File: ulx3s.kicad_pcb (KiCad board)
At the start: 4 copper layers, 94 x 50.8 mm, 222 parts, among them J1 CONN_02X20, J2 CONN_02X20, J3 WIFI_OFF, J4 CONN_02X03, J5 VJ1, Q1 BC857, Q2 2N7002, SW1 SW_DIP_x04, U1 LFE5U-85F-6BG381C, U10 IS25LP128F-JBLE, U11 PCA9306D, U2 MT48LC16M16A2TG, U3 TLV62569DBV, U4 TLV62569DBV, U5 TLV62569DBV, U6 FT231XS, U7 MCP7940NT, U8 MAX11125, U9 ESP32, Y1 FNETHE025, Y2 32768Hz

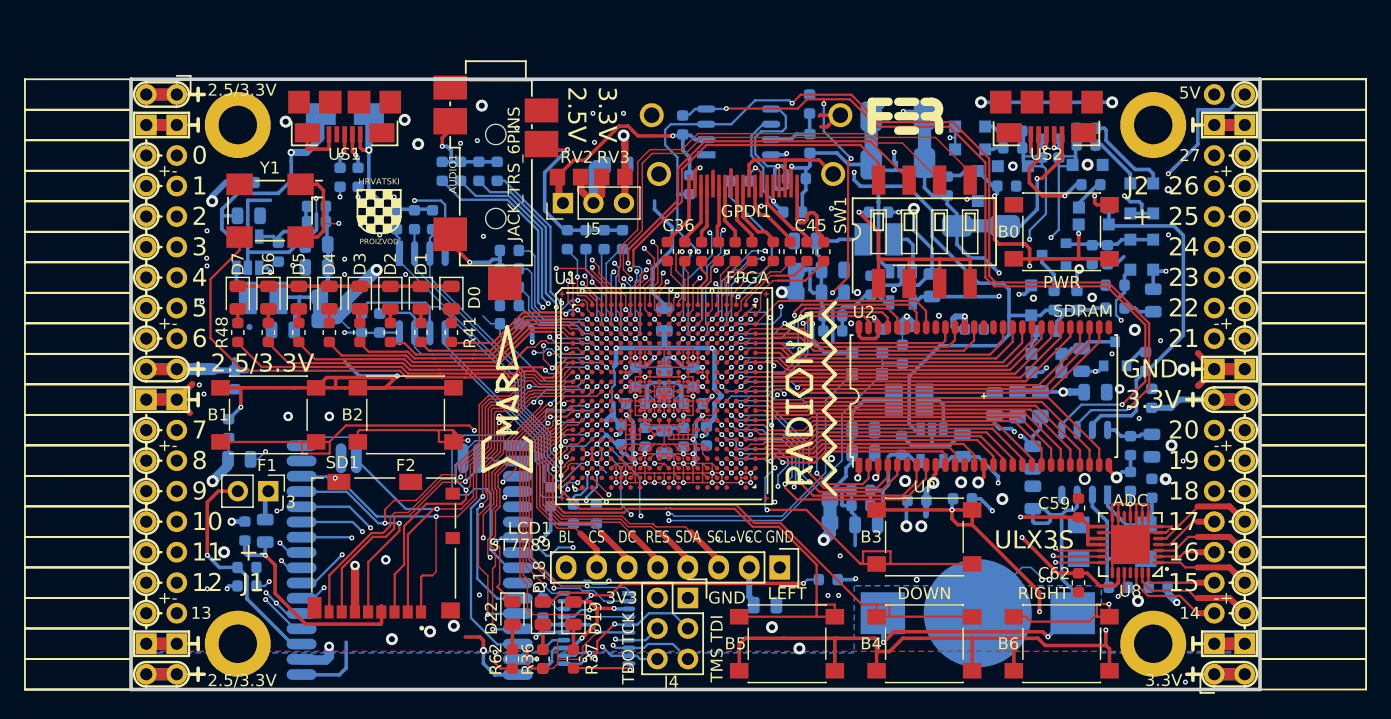
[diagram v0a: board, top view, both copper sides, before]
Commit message: First pass cleanup
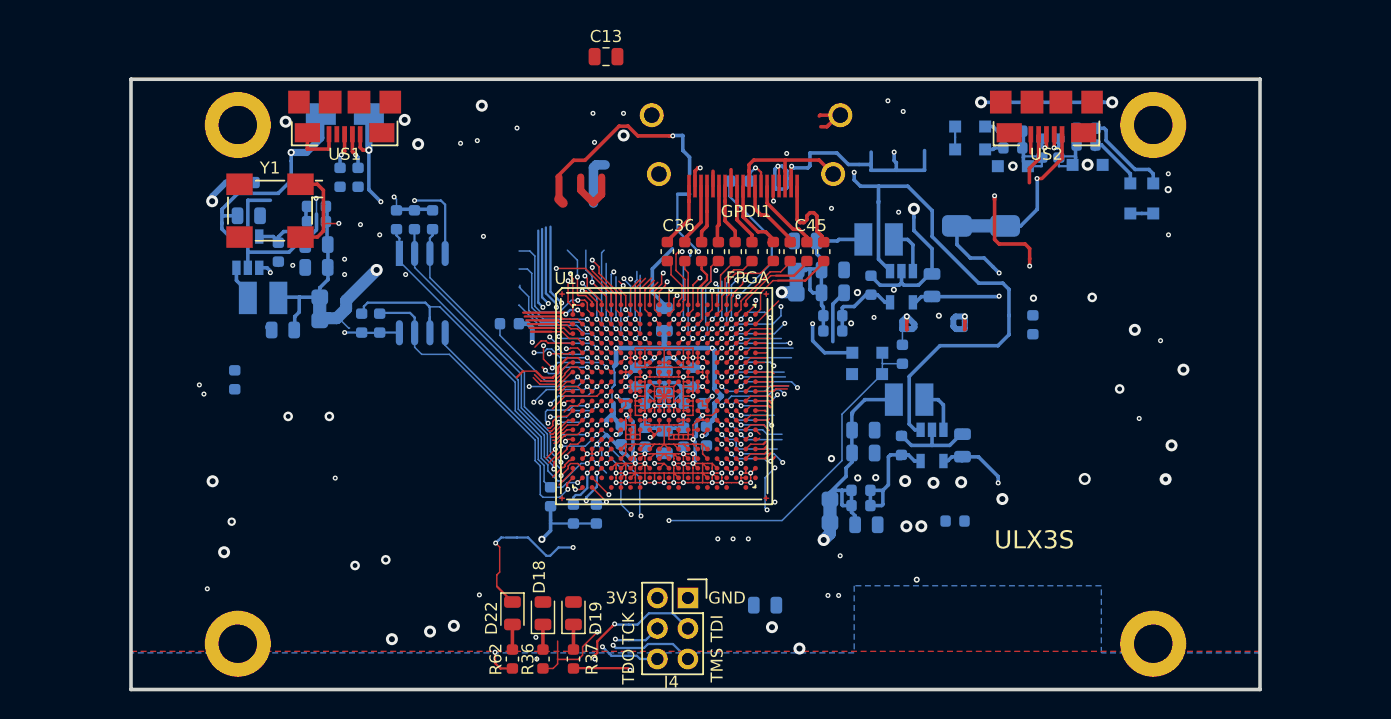
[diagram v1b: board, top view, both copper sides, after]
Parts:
- removed AE1: 433MHz, TestPoint:TestPoint_Pad_D1.0mm
- removed AUDIO1: JACK_TRS_6PINS, audio-jack:CUI_SJ-43516-SMT
- removed B0, B1, B2, B3, B4, B5, B6: PTS645, Button_Switch_SMD:SW_SPST_PTS645
- removed BAT1: CR1225, Keystone_3000_1x12mm-CoinCell:Keystone_3000_1x12mm-CoinCell
- removed C14, C59, C60, C62: 220nF, Capacitor_SMD:C_0603_1608Metric
- removed C15, C21, C54, C55, C58, C61: 22uF, Capacitor_SMD:C_0805_2012Metric
- removed C16, C47: 2.2uF, Capacitor_SMD:C_0805_2012Metric
- removed C18: 470pF, Capacitor_SMD:C_0603_1608Metric
- removed C33, C34, C35, C52: 22nF, Capacitor_SMD:C_0603_1608Metric
- removed C56, C57: 4.7pF, Capacitor_SMD:C_0603_1608Metric
- removed D0, D11, D4: RED, LED_SMD:LED_0805_2012Metric
- removed D1, D5: ORANGE, LED_SMD:LED_0805_2012Metric
- removed D10, D13, D14, D16, D17, D27: 1N914, Diode_SMD:D_SOD-323_HandSoldering
- removed D12, D15: BAT54W, Diode_SMD:D_SOD-323_HandSoldering
- removed D2, D6: GREEN, LED_SMD:LED_0805_2012Metric
- removed D3, D7: BLUE, LED_SMD:LED_0805_2012Metric
- removed D51, D52: 0, jumper:D_SMA_Jumper_NC
- removed HR: HR, hrvatski_proizvod_veci:hrvatski
- removed J1, J2: CONN_02X20, Socket_Strips:Socket_Strip_Angled_2x20
- removed J3: WIFI_OFF, Connector_PinHeader_2.54mm:PinHeader_1x02_P2.54mm_Vertical
- removed J5: VJ1, Connector_PinHeader_2.54mm:PinHeader_1x03_P2.54mm_Vertical
- removed L4, L5: 33uH, Inductor_SMD:L_0805_2012Metric_Pad1.15x1.40mm_HandSolder
- removed LCD1: ST7789, st7789:st7789
- removed Q1: BC857, Package_TO_SOT_SMD:SOT-23
- removed Q2: 2N7002, Package_TO_SOT_SMD:SOT-23
- removed R1, R25, R26, R3, R4: 4.7k, Resistor_SMD:R_0603_1608Metric
- removed R10, R17, R21, R39, R51, R60, R7: 130, Resistor_SMD:R_0603_1608Metric
- removed R13, R34, R9: 15k, Resistor_SMD:R_0603_1608Metric
- removed R14, R18, R57, R6, R66, R8: 1.1k, Resistor_SMD:R_0603_1608Metric
- removed R15, R19, R35, R41, R42, R43, R44, R45, R46, R47, R48, R58, R65: 549, Resistor_SMD:R_0603_1608Metric
- removed R16, R20, R59: 270, Resistor_SMD:R_0603_1608Metric
- removed R2: 18k, Resistor_SMD:R_0603_1608Metric
- removed R22, R23: 3.3k, Resistor_SMD:R_0603_1608Metric
- removed R24: 100k, Resistor_SMD:R_0603_1608Metric
- removed R38: 0.47, Resistor_SMD:R_0603_1608Metric
- removed R5: 2.2M, Resistor_SMD:R_0603_1608Metric
- removed R56: 0, Resistor_SMD:R_0603_1608Metric
- removed REF** (x2): emard12mm, emard:emard12mm
- removed REF**: inem, inem:inem
- removed RV2, RV3: 0, Resistor_SMD:R_0805_2012Metric_Pad1.29x1.40mm_HandSolder
- removed SD1: 104031-0811, micro-sd-104031-811:MOLEX_104031-0811
- removed SW1: SW_DIP_x04, dipswitch:SW_DIP_x4_W8.61mm_Slide_LowProfile
- removed U11: PCA9306D, SM8:SM8
- removed U2: MT48LC16M16A2TG, TSOP54:TSOP54
- removed U6: FT231XS, ft231x:FT231X-SSOP-20_4.4x6.5mm_Pitch0.65mm
- removed U7: MCP7940NT, SOT96-1:SOT96-1
- removed U8: MAX11125, max1112x-tqfn28:MAX1112x-TQFN-28-1EP_5x5mm_Pitch0.5mm
- removed U9: ESP32, ESP32:ESP32
- removed Y2: 32768Hz, abs25:Crystal_SMD_ABS25
- removed fer: fer, fer:fer
- removed koncar: koncar, koncar:koncar
- removed radiona: radiona, radiona:radiona
- C13: moved to F.Cu
- moved C13 46.9 mm to (133.6, 59.5), turned to 0 degrees
- moved C51 17.8 mm to (162.7, 98.2)
- moved C50 11.6 mm to (169.2, 81.9)
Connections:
- C13 pad 1: +5V -> GND
- C13 pad 2: /power/WKUP -> 2V5_3V3
- C20 pad 1: +3V3 -> 2V5_3V3
- C25 pad 1: +3V3 -> 2V5_3V3
- C31 pad 1: +3V3 -> 2V5_3V3
- C32 pad 1: +3V3 -> 2V5_3V3
- C46 pad 1: +3V3 -> 2V5_3V3
- C50 pad 1: +3V3 -> 2V5_3V3
- C51 pad 1: +3V3 -> 2V5_3V3
- D18 pad 2: FTDI_nSLEEP -> (no net)
- D19 pad 2: FT2V5 -> (no net)
- D28 pad 1: PWRBTn -> (no net)
- GPDI1 pad 15: GPDI_SCL -> (no net)
- GPDI1 pad 16: GPDI_SDA -> (no net)
- J4 pad 2: +3V3 -> 2V5_3V3
- R11 pad 1: +3V3 -> 2V5_3V3
- R12 pad 1: +3V3 -> 2V5_3V3
- R27 pad 1: +3V3 -> 2V5_3V3
- R28 pad 1: +3V3 -> 2V5_3V3
- R29 pad 1: +3V3 -> 2V5_3V3
- R30 pad 1: +3V3 -> 2V5_3V3
- R31 pad 1: +3V3 -> 2V5_3V3
- R32 pad 1: +3V3 -> 2V5_3V3
- R33 pad 1: +3V3 -> 2V5_3V3
- R37 pad 1: FTDI_nTXLED -> (no net)
- R49 pad 1: USB_FTDI_D- -> (no net)
- R50 pad 1: USB_FTDI_D+ -> (no net)
- R62 pad 2: +3V3 -> 2V5_3V3
- RP3 pad 2: +3V3 -> 2V5_3V3
- U1 pad A10: GP1 -> (no net)
- U1 pad A11: GN1 -> (no net)
- U1 pad A15: Net-(U1-PadA15) -> (no net)
- U1 pad A2: GP9 -> (no net)
- U1 pad A3: AUDIO_R0 -> (no net)
- U1 pad A4: GP8 -> (no net)
- U1 pad A5: GN8 -> (no net)
- U1 pad A6: GP7 -> (no net)
- U1 pad A7: GP4 -> (no net)
- U1 pad A8: GN4 -> (no net)
- U1 pad A9: GP2 -> (no net)
- U1 pad B1: GN9 -> (no net)
- U1 pad B10: GN2 -> (no net)
- U1 pad B11: GP0 -> (no net)
- U1 pad B13: GP26 -> (no net)
- U1 pad B15: GP22 -> (no net)
- U1 pad B17: GP23 -> (no net)
- U1 pad B19: FPDI_SDA -> (no net)
- U1 pad B2: LED0 -> (no net)
- U1 pad B3: AUDIO_L3 -> (no net)
- U1 pad B4: GN10 -> (no net)
- U1 pad B5: AUDIO_R1 -> (no net)
- U1 pad B6: GN7 -> (no net)
- U1 pad B8: GN5 -> (no net)
- U1 pad B9: GP3 -> (no net)
- U1 pad C1: LED2 -> (no net)
- U1 pad C10: GN3 -> (no net)
- U1 pad C11: GN0 -> (no net)
- U1 pad C13: GN26 -> (no net)
- U1 pad C15: GN22 -> (no net)
- U1 pad C16: GP24 -> (no net)
- U1 pad C17: GN23 -> (no net)
- U1 pad C18: GP21 -> (no net)
- U1 pad C2: LED1 -> (no net)
- U1 pad C20: SDRAM_D11 -> (no net)
- U1 pad C3: AUDIO_L2 -> (no net)
- U1 pad C4: GP10 -> (no net)
- U1 pad C5: AUDIO_R3 -> (no net)
- U1 pad C6: GP6 -> (no net)
- U1 pad C7: GN6 -> (no net)
- U1 pad C8: GP5 -> (no net)
- U1 pad C9: Net-(U1-PadC9) -> (no net)
- U1 pad D1: LED4 -> (no net)
- U1 pad D10: Net-(U1-PadD10) -> (no net)
- U1 pad D11: Net-(U1-PadD11) -> (no net)
- U1 pad D12: Net-(U1-PadD12) -> (no net)
- U1 pad D13: GP27 -> (no net)
- U1 pad D14: GP25 -> (no net)
- U1 pad D16: GN24 -> (no net)
- U1 pad D17: GN21 -> (no net)
- U1 pad D18: GP20 -> (no net)
- U1 pad D19: SDRAM_D10 -> (no net)
- U1 pad D2: LED3 -> (no net)
- U1 pad D20: SDRAM_D9 -> (no net)
- U1 pad D3: AUDIO_L1 -> (no net)
- U1 pad D5: AUDIO_R2 -> (no net)
- U1 pad D6: BTN_PWRn -> (no net)
- U1 pad D7: SW3 -> (no net)
- U1 pad D8: SW2 -> (no net)
- U1 pad D9: Net-(U1-PadD9) -> (no net)
- U1 pad E1: LED6 -> (no net)
- U1 pad E10: Net-(U1-PadE10) -> (no net)
- U1 pad E11: Net-(U1-PadE11) -> (no net)
- U1 pad E12: FPDI_SCL -> (no net)
- U1 pad E13: GN27 -> (no net)
- U1 pad E14: GN25 -> (no net)
- U1 pad E17: GN20 -> (no net)
- U1 pad E18: SDRAM_D12 -> (no net)
- U1 pad E19: SDRAM_D8 -> (no net)
- U1 pad E2: LED5 -> (no net)
- U1 pad E20: SDRAM_DQM1 -> (no net)
- U1 pad E3: GN11 -> (no net)
- U1 pad E4: AUDIO_L0 -> (no net)
- U1 pad E5: AUDIO_V3 -> (no net)
- U1 pad E6: WIFI_GPIO35 -> (no net)
- U1 pad E7: SW4 -> (no net)
- U1 pad E8: SW1 -> (no net)
- U1 pad E9: WIFI_GPIO25 -> (no net)
- U1 pad F1: WIFI_EN -> (no net)
- U1 pad F11: +3V3 -> 2V5_3V3
- U1 pad F12: +3V3 -> 2V5_3V3
- U1 pad F17: GP19 -> (no net)
- U1 pad F18: SDRAM_D13 -> (no net)
- U1 pad F19: SDRAM_CLK -> (no net)
- U1 pad F2: AUDIO_V1 -> (no net)
- U1 pad F20: SDRAM_CKE -> (no net)
- U1 pad F3: GN12 -> (no net)
- U1 pad F4: GP11 -> (no net)
- U1 pad F5: AUDIO_V2 -> (no net)
- U1 pad G16: SHUTDOWN -> (no net)
- U1 pad G18: GN19 -> (no net)
- U1 pad G19: SDRAM_A12 -> (no net)
- U1 pad G20: SDRAM_A11 -> (no net)
- U1 pad G3: GP12 -> (no net)
- U1 pad G5: GN13 -> (no net)
- U1 pad H1: SD_D1 -> (no net)
- U1 pad H14: +3V3 -> 2V5_3V3
- U1 pad H15: +3V3 -> 2V5_3V3
- U1 pad H16: BTN_R -> (no net)
- U1 pad H17: GN18 -> (no net)
- U1 pad H18: GP18 -> (no net)
- U1 pad H2: SD_CLK -> (no net)
- U1 pad H20: SDRAM_A9 -> (no net)
- U1 pad H3: LED7 -> (no net)
- U1 pad H4: GP13 -> (no net)
- U1 pad H5: AUDIO_V0 -> (no net)
- U1 pad J1: SD_CMD -> (no net)
- U1 pad J15: +3V3 -> 2V5_3V3
- U1 pad J16: SDRAM_D0 -> (no net)
- U1 pad J17: SDRAM_D15 -> (no net)
- U1 pad J18: SDRAM_D14 -> (no net)
- U1 pad J19: SDRAM_A8 -> (no net)
- U1 pad J20: SDRAM_A7 -> (no net)
- U1 pad J3: SD_D0 -> (no net)
- U1 pad J4: OLED_BL -> (no net)
- U1 pad J5: WIFI_GPIO22 -> (no net)
- U1 pad K1: SD_D2 -> (no net)
- U1 pad K16: Net-(U1-PadK16) -> (no net)
- U1 pad K17: Net-(U1-PadK17) -> (no net)
- U1 pad K18: SDRAM_A6 -> (no net)
- U1 pad K19: SDRAM_A5 -> (no net)
- U1 pad K2: SD_D3 -> (no net)
- U1 pad K20: SDRAM_A4 -> (no net)
- U1 pad K3: WIFI_RXD -> (no net)
- U1 pad K4: WIFI_TXD -> (no net)
- U1 pad K5: WIFI_GPIO21 -> (no net)
- U1 pad L1: WIFI_GPIO26 -> (no net)
- U1 pad L14: +3V3 -> 2V5_3V3
- U1 pad L15: +3V3 -> 2V5_3V3
- U1 pad L16: GP17 -> (no net)
- U1 pad L17: GN17 -> (no net)
- U1 pad L18: SDRAM_D1 -> (no net)
- U1 pad L19: SDRAM_A3 -> (no net)
- U1 pad L2: WIFI_GPIO0 -> (no net)
- U1 pad L20: SDRAM_A2 -> (no net)
- U1 pad L3: FTDI_TXDEN -> (no net)
- U1 pad L4: FTDI_RXD -> (no net)
- U1 pad L5: FTDI_nRXLED -> (no net)
- U1 pad L6: +3V3 -> 2V5_3V3
- U1 pad L7: +3V3 -> 2V5_3V3
- U1 pad M1: FTDI_TXD -> (no net)
- U1 pad M15: +3V3 -> 2V5_3V3
- U1 pad M17: GN16 -> (no net)
- U1 pad M18: SDRAM_D2 -> (no net)
- U1 pad M19: SDRAM_A1 -> (no net)
- U1 pad M20: SDRAM_A0 -> (no net)
- U1 pad M3: FTDI_nRTS -> (no net)
- U1 pad M5: Net-(U1-PadM5) -> (no net)
- U1 pad M6: +3V3 -> 2V5_3V3
- U1 pad N1: FTDI_nDTR -> (no net)
- U1 pad N16: GP16 -> (no net)
- U1 pad N17: GP15 -> (no net)
- U1 pad N18: SDRAM_D3 -> (no net)
- U1 pad N19: SDRAM_A10 -> (no net)
- U1 pad N2: OLED_CS -> (no net)
- U1 pad N20: SDRAM_BA1 -> (no net)
- U1 pad N3: WIFI_GPIO27 -> (no net)
- U1 pad N4: WIFI_GPIO19 -> (no net)
- U1 pad N5: SD_CD -> (no net)
- U1 pad P1: OLED_DC -> (no net)
- U1 pad P10: +3V3 -> 2V5_3V3
- U1 pad P16: GN15 -> (no net)
- U1 pad P17: ADC_SCLK -> (no net)
- U1 pad P18: SDRAM_D4 -> (no net)
- U1 pad P19: SDRAM_BA0 -> (no net)
- U1 pad P2: OLED_RES -> (no net)
- U1 pad P20: SDRAM_nCS -> (no net)
- U1 pad P3: OLED_MOSI -> (no net)
- U1 pad P4: OLED_CLK -> (no net)
- U1 pad P5: SD_WP -> (no net)
- U1 pad P9: +3V3 -> 2V5_3V3
- U1 pad R1: BTN_F1 -> (no net)
- U1 pad R16: ADC_MOSI -> (no net)
- U1 pad R17: ADC_CSn -> (no net)
- U1 pad R18: BTN_U -> (no net)
- U1 pad R20: SDRAM_nRAS -> (no net)
- U1 pad R3: Net-(U1-PadR3) -> (no net)
- U1 pad T1: BTN_F2 -> (no net)
- U1 pad T16: Net-(U1-PadT16) -> (no net)
- U1 pad T17: SDRAM_D6 -> (no net)
- U1 pad T18: SDRAM_D5 -> (no net)
- U1 pad T19: SDRAM_nCAS -> (no net)
- U1 pad T2: +3V3 -> 2V5_3V3
- U1 pad T20: SDRAM_nWE -> (no net)
- U1 pad T3: +3V3 -> 2V5_3V3
- U1 pad T4: +3V3 -> 2V5_3V3
- U1 pad U1: BTN_L -> (no net)
- U1 pad U16: ADC_MISO -> (no net)
- U1 pad U17: GN14 -> (no net)
- U1 pad U18: GP14 -> (no net)
- U1 pad U19: SDRAM_DQM0 -> (no net)
- U1 pad U2: +3V3 -> 2V5_3V3
- U1 pad U20: SDRAM_D7 -> (no net)
- U1 pad V1: BTN_D -> (no net)
- U1 pad W13: Net-(U1-PadW13) -> (no net)
- U1 pad W14: Net-(U1-PadW14) -> (no net)
- U1 pad W17: Net-(U1-PadW17) -> (no net)
- U1 pad W18: Net-(U1-PadW18) -> (no net)
- U1 pad W20: Net-(U1-PadW20) -> (no net)
- U1 pad W4: Net-(U1-PadW4) -> (no net)
- U1 pad W5: Net-(U1-PadW5) -> (no net)
- U1 pad W8: Net-(U1-PadW8) -> (no net)
- U1 pad W9: Net-(U1-PadW9) -> (no net)
- U1 pad Y11: Net-(U1-PadY11) -> (no net)
- U1 pad Y12: Net-(U1-PadY12) -> (no net)
- U1 pad Y14: Net-(U1-PadY14) -> (no net)
- U1 pad Y15: Net-(U1-PadY15) -> (no net)
- U1 pad Y16: Net-(U1-PadY16) -> (no net)
- U1 pad Y17: Net-(U1-PadY17) -> (no net)
- U1 pad Y19: Net-(U1-PadY19) -> (no net)
- U1 pad Y5: Net-(U1-PadY5) -> (no net)
- U1 pad Y6: Net-(U1-PadY6) -> (no net)
- U1 pad Y7: Net-(U1-PadY7) -> (no net)
- U1 pad Y8: Net-(U1-PadY8) -> (no net)
- U10 pad 8: +3V3 -> 2V5_3V3
- U3 pad 1: /power/PWREN -> +5V
- U4 pad 1: /power/PWREN -> +5V
- U5 pad 1: /power/PWREN -> +5V
- US1 pad 4: Net-(US1-Pad4) -> (no net)
- US2 pad 4: US2_ID -> (no net)
- Y1 pad 1: +3V3 -> 2V5_3V3
- Y1 pad 4: +3V3 -> 2V5_3V3
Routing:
- net (no net): track 0.00 -> 834.9 mm, vias 0 -> 160
- net +3V3: track 184.1 -> 0.00 mm, vias 33 -> 0
- net GND: track 458.6 -> 304.4 mm, vias 136 -> 124
- net /power/PWREN: track 115.6 -> 0.00 mm, vias 3 -> 0
- net /usb/ANT_433MHz: track 111.7 -> 4.23 mm, vias 2 -> 0
- net FPDI_SDA: track 91.9 -> 0.00 mm, vias 6 -> 0
- net FPDI_SCL: track 89.0 -> 0.00 mm, vias 4 -> 0
- net +5V: track 149.0 -> 233.3 mm, vias 7 -> 9
- net /blinkey/BTNPUR: track 76.6 -> 0.00 mm, vias 3 -> 0
- net BTN_R: track 70.5 -> 0.00 mm, vias 4 -> 0
- net GP15: track 58.6 -> 0.00 mm, vias 2 -> 0
- net USB_FTDI_D+: track 58.5 -> 0.00 mm, vias 2 -> 0
- net GP14: track 58.1 -> 0.00 mm, vias 1 -> 0
- net GP17: track 58.0 -> 0.00 mm, vias 2 -> 0
- net GP16: track 57.0 -> 0.00 mm, vias 1 -> 0
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- removed copper zone on In1.Cu, net +3V3
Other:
- board text removed: "+-"
- board text removed: "-+"
- board text removed: "0"
- board text removed: "1"
- board text removed: "10"
- board text removed: "11"
- board text removed: "12"
- board text removed: "13"
- board text removed: "14"
- board text removed: "15"
- board text removed: "16"
- board text removed: "17"
- board text removed: "18"
- board text removed: "19"
- board text removed: "2"
- board text removed: "2.5/3.3V"
- board text removed: "2.5V"
- board text removed: "20"
- board text removed: "21"
- board text removed: "22"
- board text removed: "23"
- board text removed: "24"
- board text removed: "25"
- board text removed: "26"
- board text removed: "27"
- board text removed: "3"
- board text removed: "3.3V"
- board text removed: "3V 12.5x2.5mm"
- board text removed: "4"
- board text removed: "5"
- board text removed: "5V"
- board text removed: "6"
- board text removed: "7"
- board text removed: "8"
- board text removed: "9"
- board text removed: "ADC"
- board text removed: "CR1225"
- board text removed: "DOWN"
- board text removed: "F1"
- board text removed: "F2"
- board text removed: "LEFT"
- board text removed: "PWR"
- board text removed: "RIGHT"
- board text removed: "RTC"
- board text removed: "SDRAM"
- board text removed: "UP"
- board text removed: "skriptarnica.hr"
